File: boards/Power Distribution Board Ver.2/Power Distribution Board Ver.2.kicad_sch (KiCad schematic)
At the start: 90 parts, among them J1 Screw_Terminal_01x02, J2 Screw_Terminal_01x06, J3 Screw_Terminal_01x06, J5 Screw_Terminal_01x06, J6 USB_A, K1 Relay, K2 Relay, K3 Relay, K4 Relay, K5 Relay, K6 Relay, SW1 SW_Push_Open, U1 SIC431AED-T1-GE3, U2 SIC431AED-T1-GE3, U3 SIC431AED-T1-GE3

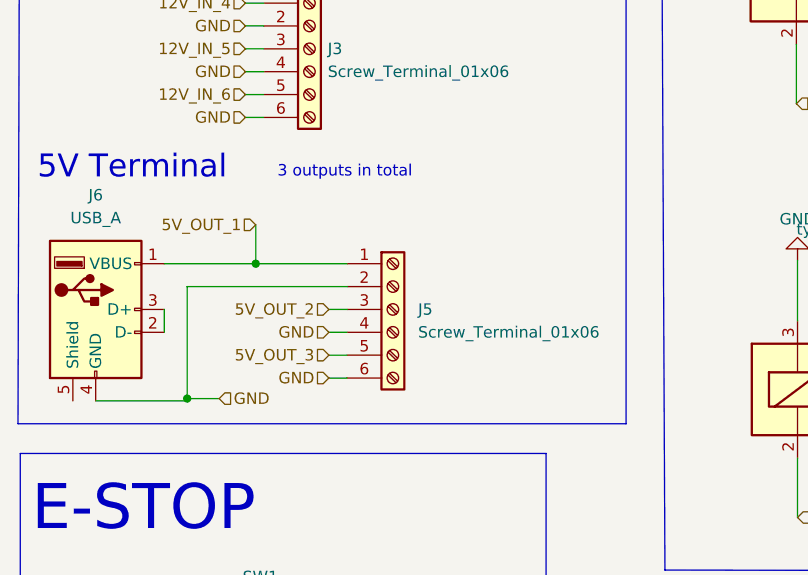
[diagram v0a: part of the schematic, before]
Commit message: Add Positive
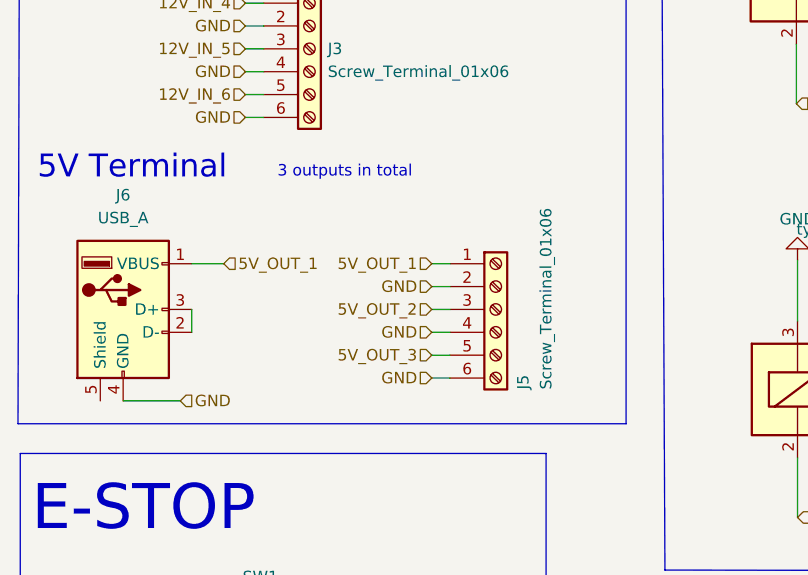
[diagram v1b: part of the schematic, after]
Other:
- moved on the sheet: J5, J6
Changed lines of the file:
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@@
   (junction (at 144.78 253.492) (diameter 0) (color 0 0 0 0)
   )
-  (junction (at 32.512 101.346) (diameter 0) (color 0 0 0 0)
-  )
   (junction (at 144.526 191.516) (diameter 0) (color 0 0 0 0)
   )
@@
   (junction (at 183.007 196.723) (diameter 0) (color 0 0 0 0)
   )
-  (junction (at 40.132 86.36) (diameter 0) (color 0 0 0 0)
-  )
   (wire (pts (xy 58.801 209.296) (xy 58.801 209.931))
     (stroke (width 0) (type default))
@@
     (stroke (width 0) (type default))
   )
-  (wire (pts (xy 48.26 99.06) (xy 50.292 99.06))
+  (wire (pts (xy 59.69 99.06) (xy 61.722 99.06))
     (stroke (width 0) (type default))
   )
@@
     (stroke (width 0) (type default))
   )
-  (wire (pts (xy 32.512 88.9) (xy 32.512 101.346))
-    (stroke (width 0) (type default))
-  )
   (wire (pts (xy 38.862 32.004) (xy 40.767 32.004))
     (stroke (width 0) (type default))
@@
     (stroke (width 0) (type default))
   )
-  (wire (pts (xy 50.292 88.9) (xy 32.512 88.9))
-    (stroke (width 0) (type default))
-  )
   (wire (pts (xy 59.055 241.427) (xy 59.055 248.412))
     (stroke (width 0) (type default))
@@
     (stroke (width 0) (type default))
   )
-  (wire (pts (xy 32.512 101.6) (xy 22.352 101.6))
-    (stroke (width 0) (type default))
-  )
   (wire (pts (xy 192.278 234.188) (xy 192.278 236.728))
     (stroke (width 0) (type default))
@@
     (stroke (width 0) (type default))
   )
-  (wire (pts (xy 32.512 101.346) (xy 36.068 101.346))
-    (stroke (width 0) (type default))
-  )
   (wire (pts (xy 172.847 172.593) (xy 183.007 172.593))
     (stroke (width 0) (type default))
@@
     (stroke (width 0) (type default))
   )
-  (wire (pts (xy 29.972 86.36) (xy 40.132 86.36))
-    (stroke (width 0) (type default))
-  )
   (polyline (pts (xy 16.764 136.652) (xy 240.284 136.652))
     (stroke (width 0) (type default))
@@
     (stroke (width 0) (type default))
   )
-  (wire (pts (xy 40.132 86.36) (xy 50.292 86.36))
-    (stroke (width 0) (type default))
-  )
   (wire (pts (xy 59.055 271.272) (xy 59.055 271.907))
     (stroke (width 0) (type default))
@@
     (stroke (width 0) (type default))
   )
+  (wire (pts (xy 25.4 101.6) (xy 31.75 101.6))
+    (stroke (width 0) (type default))
+  )
   (wire (pts (xy 195.707 172.593) (xy 202.057 172.593))
     (stroke (width 0) (type default))
@@
     (stroke (width 0) (type default))
   )
+  (wire (pts (xy 59.69 86.36) (xy 61.722 86.36))
+    (stroke (width 0) (type default))
+  )
   (wire (pts (xy 59.055 248.412) (xy 97.79 248.412))
     (stroke (width 0) (type default))
@@
     (stroke (width 0) (type default))
   )
-  (wire (pts (xy 48.26 91.44) (xy 50.292 91.44))
+  (wire (pts (xy 59.69 91.44) (xy 61.722 91.44))
     (stroke (width 0) (type default))
   )
@@
     (stroke (width 0) (type default))
   )
-  (wire (pts (xy 32.512 101.346) (xy 32.512 101.6))
-    (stroke (width 0) (type default))
-  )
   (wire (pts (xy 177.546 42.418) (xy 177.546 47.752))
     (stroke (width 0) (type default))
@@
     (stroke (width 0) (type default))
   )
-  (wire (pts (xy 29.972 91.44) (xy 29.972 93.98))
+  (wire (pts (xy 33.02 91.44) (xy 33.02 93.98))
     (stroke (width 0) (type default))
   )
@@
     (stroke (width 0) (type default))
   )
+  (wire (pts (xy 33.02 86.36) (xy 36.576 86.36))
+    (stroke (width 0) (type default))
+  )
   (wire (pts (xy 133.35 234.442) (xy 147.955 234.442))
     (stroke (width 0) (type default))
@@
     (stroke (width 0) (type default))
   )
-  (wire (pts (xy 48.26 93.98) (xy 50.292 93.98))
+  (wire (pts (xy 59.69 93.98) (xy 61.722 93.98))
     (stroke (width 0) (type default))
   )
@@
     (stroke (width 0) (type default))
   )
-  (wire (pts (xy 48.26 96.52) (xy 50.292 96.52))
+  (wire (pts (xy 59.69 96.52) (xy 61.722 96.52))
     (stroke (width 0) (type default))
   )
@@
     (stroke (width 0) (type default))
   )
-  (wire (pts (xy 40.132 82.042) (xy 40.132 86.36))
-    (stroke (width 0) (type default))
-  )
   (polyline (pts (xy 13.716 13.97) (xy 81.28 13.97))
     (stroke (width 0) (type default))
   )
   (wire (pts (xy 202.057 196.723) (xy 208.407 196.723))
+    (stroke (width 0) (type default))
+  )
+  (wire (pts (xy 59.69 88.9) (xy 61.722 88.9))
     (stroke (width 0) (type default))
   )
@@
     (effects (font (size 1.27 1.27)) (justify left))
   )
-  (hierarchical_label "5V_OUT_1" (shape input) (at 40.132 82.042 180) (fields_autoplaced)
+  (hierarchical_label "5V_OUT_1" (shape input) (at 59.69 86.36 180) (fields_autoplaced)
     (effects (font (size 1.27 1.27)) (justify right))
   )
@@
     (effects (font (size 1.27 1.27)) (justify left))
   )
-  (hierarchical_label "GND" (shape input) (at 48.26 99.06 180) (fields_autoplaced)
+  (hierarchical_label "GND" (shape input) (at 59.69 99.06 180) (fields_autoplaced)
     (effects (font (size 1.27 1.27)) (justify right))
   )
@@
     (effects (font (size 1.27 1.27)) (justify left))
   )
-  (hierarchical_label "5V_OUT_2" (shape input) (at 48.26 91.44 180) (fields_autoplaced)
+  (hierarchical_label "5V_OUT_2" (shape input) (at 59.69 91.44 180) (fields_autoplaced)
     (effects (font (size 1.27 1.27)) (justify right))
   )
@@
     (effects (font (size 1.27 1.27)) (justify left))
   )
-  (hierarchical_label "5V_OUT_3" (shape input) (at 48.26 96.52 180) (fields_autoplaced)
+  (hierarchical_label "5V_OUT_3" (shape input) (at 59.69 96.52 180) (fields_autoplaced)
     (effects (font (size 1.27 1.27)) (justify right))
   )
@@
     (effects (font (size 1.27 1.27)) (justify left))
   )
+  (hierarchical_label "GND" (shape input) (at 59.69 88.9 180) (fields_autoplaced)
+    (effects (font (size 1.27 1.27)) (justify right))
+  )
   (hierarchical_label "12V_IN_6" (shape output) (at 196.596 85.852 0) (fields_autoplaced)
     (effects (font (size 1.27 1.27)) (justify left))
@@
     (effects (font (size 1.27 1.27)) (justify right))
   )
-  (hierarchical_label "GND" (shape input) (at 48.26 93.98 180) (fields_autoplaced)
+  (hierarchical_label "GND" (shape input) (at 59.69 93.98 180) (fields_autoplaced)
     (effects (font (size 1.27 1.27)) (justify right))
   )
@@
     (effects (font (size 1.27 1.27)) (justify right))
   )
-  (hierarchical_label "GND" (shape input) (at 36.068 101.346 0) (fields_autoplaced)
+  (hierarchical_label "GND" (shape input) (at 31.75 101.6 0) (fields_autoplaced)
     (effects (font (size 1.27 1.27)) (justify left))
   )
   (hierarchical_label "12V_IN_4" (shape output) (at 119.38 86.36 0) (fields_autoplaced)
+    (effects (font (size 1.27 1.27)) (justify left))
+  )
+  (hierarchical_label "5V_OUT_1" (shape input) (at 36.576 86.36 0) (fields_autoplaced)
     (effects (font (size 1.27 1.27)) (justify left))
   )
@@
     )
   )
-  (symbol (lib_id "Connector:USB_A") (at 22.352 91.44 0) (unit 1)
+  (symbol (lib_id "Connector:USB_A") (at 25.4 91.44 0) (unit 1)
     (in_bom yes) (on_board yes) (dnp no) (fields_autoplaced)
-    (property "Reference" "J6" (at 22.352 78.74 0)
-      (effects (font (size 1.27 1.27)))
-    )
-    (property "Value" "USB_A" (at 22.352 81.28 0)
-      (effects (font (size 1.27 1.27)))
-    )
-    (property "Footprint" "Connector_USB:USB_A_CNCTech_1001-011-01101_Horizontal" (at 26.162 92.71 0)
-      (effects (font (size 1.27 1.27)) hide)
-    )
-    (property "Datasheet" " ~" (at 26.162 92.71 0)
+    (property "Reference" "J6" (at 25.4 78.74 0)
+      (effects (font (size 1.27 1.27)))
+    )
+    (property "Value" "USB_A" (at 25.4 81.28 0)
+      (effects (font (size 1.27 1.27)))
+    )
+    (property "Footprint" "Connector_USB:USB_A_CNCTech_1001-011-01101_Horizontal" (at 29.21 92.71 0)
+      (effects (font (size 1.27 1.27)) hide)
+    )
+    (property "Datasheet" "https://tools.molex.com/pdm_docs/sd/676433910_sd.pdf" (at 29.21 92.71 0)
       (effects (font (size 1.27 1.27)) hide)
     )
@@
     )
   )
-  (symbol (lib_id "Connector:Screw_Terminal_01x06") (at 55.372 91.44 0) (unit 1)
-    (in_bom yes) (on_board yes) (dnp no) (fields_autoplaced)
-    (property "Reference" "J5" (at 58.166 91.4399 0)
-      (effects (font (size 1.27 1.27)) (justify left))
-    )
-    (property "Value" "Screw_Terminal_01x06" (at 58.166 93.9799 0)
-      (effects (font (size 1.27 1.27)) (justify left))
-    )
-    (property "Footprint" "power_board_support:691137710006" (at 55.372 91.44 0)
-      (effects (font (size 1.27 1.27)) hide)
-    )
-    (property "Datasheet" "https://www.digikey.com/en/products/detail/w%C3%BCrth-elektronik/691137710006/6644055" (at 55.372 91.44 0)
-      (effects (font (size 1.27 1.27)) hide)
-    )
+  (symbol (lib_id "Connector:Screw_Terminal_01x06") (at 66.802 91.44 0) (unit 1)
+    (in_bom yes) (on_board yes) (dnp no)
+    (property "Reference" "J5" (at 69.85 100.33 90)
+      (effects (font (size 1.27 1.27)) (justify left))
+    )
+    (property "Value" "Screw_Terminal_01x06" (at 72.39 100.33 90)
+      (effects (font (size 1.27 1.27)) (justify left))
+    )
+    (property "Footprint" "power_board_support:691137710006" (at 66.802 91.44 0)
+      (effects (font (size 1.27 1.27)) hide)
+    )
+    (property "Datasheet" "https://www.digikey.com/en/products/detail/w%C3%BCrth-elektronik/691137710006/6644055" (at 66.802 91.44 0)
+      (effects (font (size 1.27 1.27)) hide)
+    )

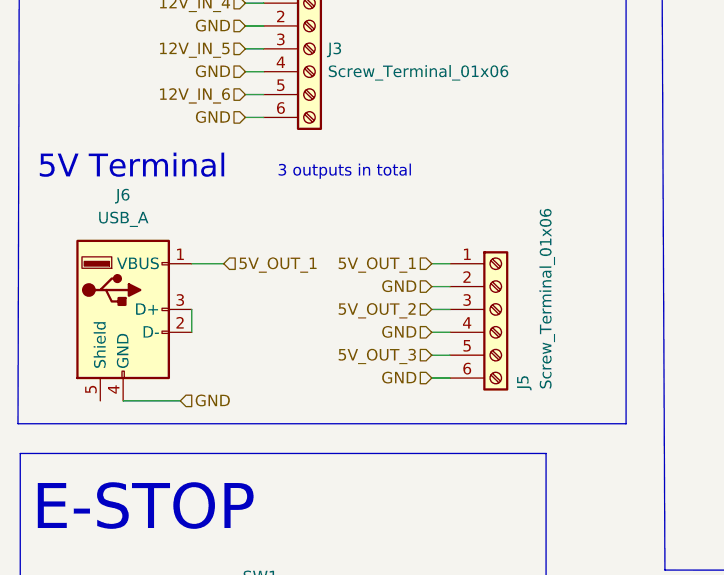
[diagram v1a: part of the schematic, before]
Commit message: Remove USB Connector
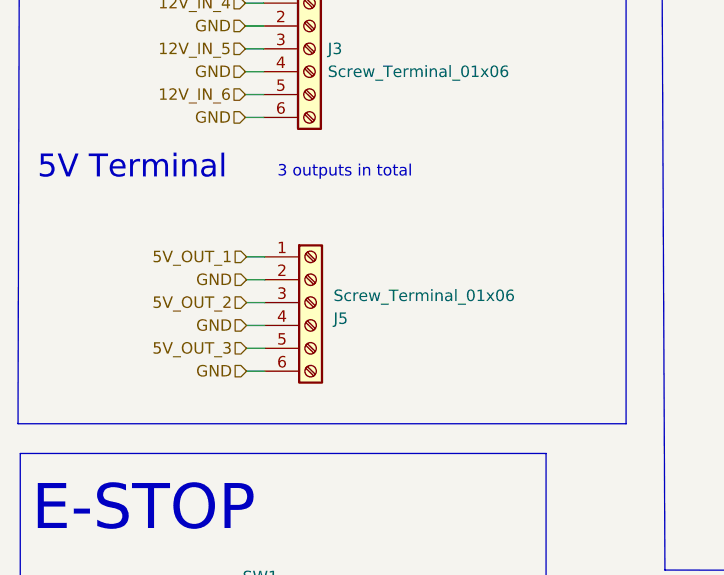
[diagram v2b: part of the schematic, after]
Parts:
- removed J6: USB_A, Connector_USB:USB_A_CNCTech_1001-011-01101_Horizontal, symbol Connector:USB_A
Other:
- moved on the sheet: J5
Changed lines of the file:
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@@
     (stroke (width 0) (type default))
   )
-  (wire (pts (xy 59.69 99.06) (xy 61.722 99.06))
+  (wire (pts (xy 39.116 98.298) (xy 41.148 98.298))
     (stroke (width 0) (type default))
   )
@@
     (stroke (width 0) (type default))
   )
-  (wire (pts (xy 25.4 101.6) (xy 31.75 101.6))
-    (stroke (width 0) (type default))
-  )
   (wire (pts (xy 195.707 172.593) (xy 202.057 172.593))
     (stroke (width 0) (type default))
@@
     (stroke (width 0) (type default))
   )
-  (wire (pts (xy 59.69 86.36) (xy 61.722 86.36))
+  (wire (pts (xy 39.116 85.598) (xy 41.148 85.598))
     (stroke (width 0) (type default))
   )
@@
     (stroke (width 0) (type default))
   )
-  (wire (pts (xy 59.69 91.44) (xy 61.722 91.44))
+  (wire (pts (xy 39.116 90.678) (xy 41.148 90.678))
     (stroke (width 0) (type default))
   )
@@
     (stroke (width 0) (type default))
   )
-  (wire (pts (xy 33.02 91.44) (xy 33.02 93.98))
-    (stroke (width 0) (type default))
-  )
   (wire (pts (xy 98.044 323.85) (xy 90.424 323.85))
     (stroke (width 0) (type default))
@@
     (stroke (width 0) (type default))
   )
-  (wire (pts (xy 33.02 86.36) (xy 36.576 86.36))
-    (stroke (width 0) (type default))
-  )
   (wire (pts (xy 133.35 234.442) (xy 147.955 234.442))
     (stroke (width 0) (type default))
@@
     (stroke (width 0) (type default))
   )
-  (wire (pts (xy 59.69 93.98) (xy 61.722 93.98))
+  (wire (pts (xy 39.116 93.218) (xy 41.148 93.218))
     (stroke (width 0) (type default))
   )
@@
     (stroke (width 0) (type default))
   )
-  (wire (pts (xy 59.69 96.52) (xy 61.722 96.52))
+  (wire (pts (xy 39.116 95.758) (xy 41.148 95.758))
     (stroke (width 0) (type default))
   )
@@
     (stroke (width 0) (type default))
   )
-  (wire (pts (xy 59.69 88.9) (xy 61.722 88.9))
+  (wire (pts (xy 39.116 88.138) (xy 41.148 88.138))
     (stroke (width 0) (type default))
   )
@@
     (effects (font (size 1.27 1.27)) (justify left))
   )
-  (hierarchical_label "5V_OUT_1" (shape input) (at 59.69 86.36 180) (fields_autoplaced)
+  (hierarchical_label "5V_OUT_1" (shape input) (at 39.116 85.598 180) (fields_autoplaced)
     (effects (font (size 1.27 1.27)) (justify right))
   )
@@
     (effects (font (size 1.27 1.27)) (justify left))
   )
-  (hierarchical_label "GND" (shape input) (at 59.69 99.06 180) (fields_autoplaced)
+  (hierarchical_label "GND" (shape input) (at 39.116 98.298 180) (fields_autoplaced)
     (effects (font (size 1.27 1.27)) (justify right))
   )
@@
     (effects (font (size 1.27 1.27)) (justify left))
   )
-  (hierarchical_label "5V_OUT_2" (shape input) (at 59.69 91.44 180) (fields_autoplaced)
+  (hierarchical_label "5V_OUT_2" (shape input) (at 39.116 90.678 180) (fields_autoplaced)
     (effects (font (size 1.27 1.27)) (justify right))
   )
@@
     (effects (font (size 1.27 1.27)) (justify left))
   )
-  (hierarchical_label "5V_OUT_3" (shape input) (at 59.69 96.52 180) (fields_autoplaced)
+  (hierarchical_label "5V_OUT_3" (shape input) (at 39.116 95.758 180) (fields_autoplaced)
     (effects (font (size 1.27 1.27)) (justify right))
   )
@@
     (effects (font (size 1.27 1.27)) (justify left))
   )
-  (hierarchical_label "GND" (shape input) (at 59.69 88.9 180) (fields_autoplaced)
+  (hierarchical_label "GND" (shape input) (at 39.116 88.138 180) (fields_autoplaced)
     (effects (font (size 1.27 1.27)) (justify right))
   )
@@
     (effects (font (size 1.27 1.27)) (justify right))
   )
-  (hierarchical_label "GND" (shape input) (at 59.69 93.98 180) (fields_autoplaced)
+  (hierarchical_label "GND" (shape input) (at 39.116 93.218 180) (fields_autoplaced)
     (effects (font (size 1.27 1.27)) (justify right))
   )
@@
     (effects (font (size 1.27 1.27)) (justify right))
   )
-  (hierarchical_label "GND" (shape input) (at 31.75 101.6 0) (fields_autoplaced)
-    (effects (font (size 1.27 1.27)) (justify left))
-  )
   (hierarchical_label "12V_IN_4" (shape output) (at 119.38 86.36 0) (fields_autoplaced)
-    (effects (font (size 1.27 1.27)) (justify left))
-  )
-  (hierarchical_label "5V_OUT_1" (shape input) (at 36.576 86.36 0) (fields_autoplaced)
     (effects (font (size 1.27 1.27)) (justify left))
   )
@@
         (path "/549cd60f-46dc-43a0-b7a0-227d65d2c004"
           (reference "C103") (unit 1)
-        )
-      )
-    )
-  )
-  (symbol (lib_id "Connector:USB_A") (at 25.4 91.44 0) (unit 1)
-    (in_bom yes) (on_board yes) (dnp no) (fields_autoplaced)
-    (property "Reference" "J6" (at 25.4 78.74 0)
-      (effects (font (size 1.27 1.27)))
-    )
-    (property "Value" "USB_A" (at 25.4 81.28 0)
-      (effects (font (size 1.27 1.27)))
-    )
-    (property "Footprint" "Connector_USB:USB_A_CNCTech_1001-011-01101_Horizontal" (at 29.21 92.71 0)
-      (effects (font (size 1.27 1.27)) hide)
-    )
-    (property "Datasheet" "https://tools.molex.com/pdm_docs/sd/676433910_sd.pdf" (at 29.21 92.71 0)
-      (effects (font (size 1.27 1.27)) hide)
-    )
-    (pin "1")
-    (pin "2")
-    (pin "3")
-    (pin "4")
-    (pin "5")
-    (instances
-      (project "Power Distribution Board Ver.2"
-        (path "/0d23e29d-c6b1-4207-83a7-2186dcec997d"
-          (reference "J6") (unit 1)
         )
       )
@@
     )
   )
-  (symbol (lib_id "Connector:Screw_Terminal_01x06") (at 66.802 91.44 0) (unit 1)
+  (symbol (lib_id "Connector:Screw_Terminal_01x06") (at 46.228 90.678 0) (unit 1)
     (in_bom yes) (on_board yes) (dnp no)
-    (property "Reference" "J5" (at 69.85 100.33 90)
-      (effects (font (size 1.27 1.27)) (justify left))
-    )
-    (property "Value" "Screw_Terminal_01x06" (at 72.39 100.33 90)
-      (effects (font (size 1.27 1.27)) (justify left))
-    )
-    (property "Footprint" "power_board_support:691137710006" (at 66.802 91.44 0)
-      (effects (font (size 1.27 1.27)) hide)
-    )
-    (property "Datasheet" "https://www.digikey.com/en/products/detail/w%C3%BCrth-elektronik/691137710006/6644055" (at 66.802 91.44 0)
-      (effects (font (size 1.27 1.27)) hide)
-    )
+    (property "Reference" "J5" (at 48.768 92.456 0)
+      (effects (font (size 1.27 1.27)) (justify left))
+    )
+    (property "Value" "Screw_Terminal_01x06" (at 48.768 89.916 0)
+      (effects (font (size 1.27 1.27)) (justify left))
+    )
+    (property "Footprint" "power_board_support:691137710006" (at 46.228 90.678 0)
+      (effects (font (size 1.27 1.27)) hide)
+    )
+    (property "Datasheet" "https://www.digikey.com/en/products/detail/w%C3%BCrth-elektronik/691137710006/6644055" (at 46.228 90.678 0)
+      (effects (font (size 1.27 1.27)) hide)
+    )
